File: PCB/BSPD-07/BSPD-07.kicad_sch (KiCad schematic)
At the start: 66 parts, among them IC1 LM393LVQDRQ1, IC2 LM393LVQDRQ1, IC3 LM393LVQDRQ1, IC4 LDO40LPU50RY, IC5 74LVC1G02GW-Q100H, IC6 LM393LVQDRQ1, J1 DTM13-12PA, Q1 RSQ025P03HZGTR, Q2 RJU002N06FRAT106, Q3 RJU002N06FRAT106, Q4 AO3401A, U2 TLP175A / COMUS AB38-Q

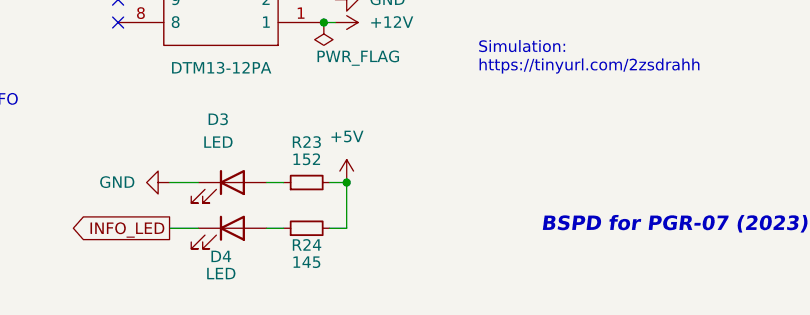
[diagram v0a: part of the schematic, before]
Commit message: Minor changes after assembly
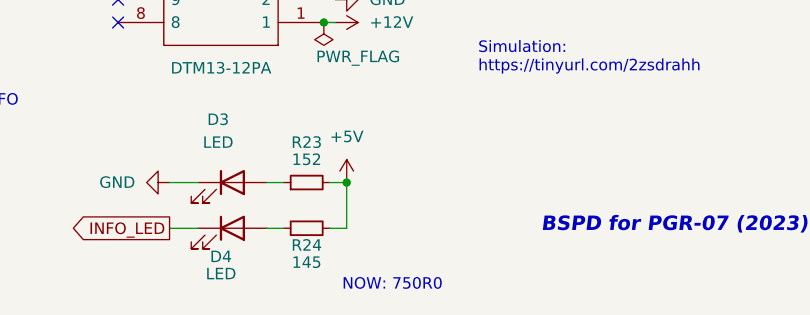
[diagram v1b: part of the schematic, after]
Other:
- note added: "NOW: 750R0"
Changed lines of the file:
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@@
     (effects (font (size 1.8 1.8)) (justify left bottom))
+  )
+  (text "NOW: 750R0" (at 163.957 217.297 0)
+    (effects (font (size 1.27 1.27)) (justify left bottom))
   )
   (text "LDO" (at 212.09 104.14 0)
